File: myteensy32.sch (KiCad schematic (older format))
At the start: 2 parts

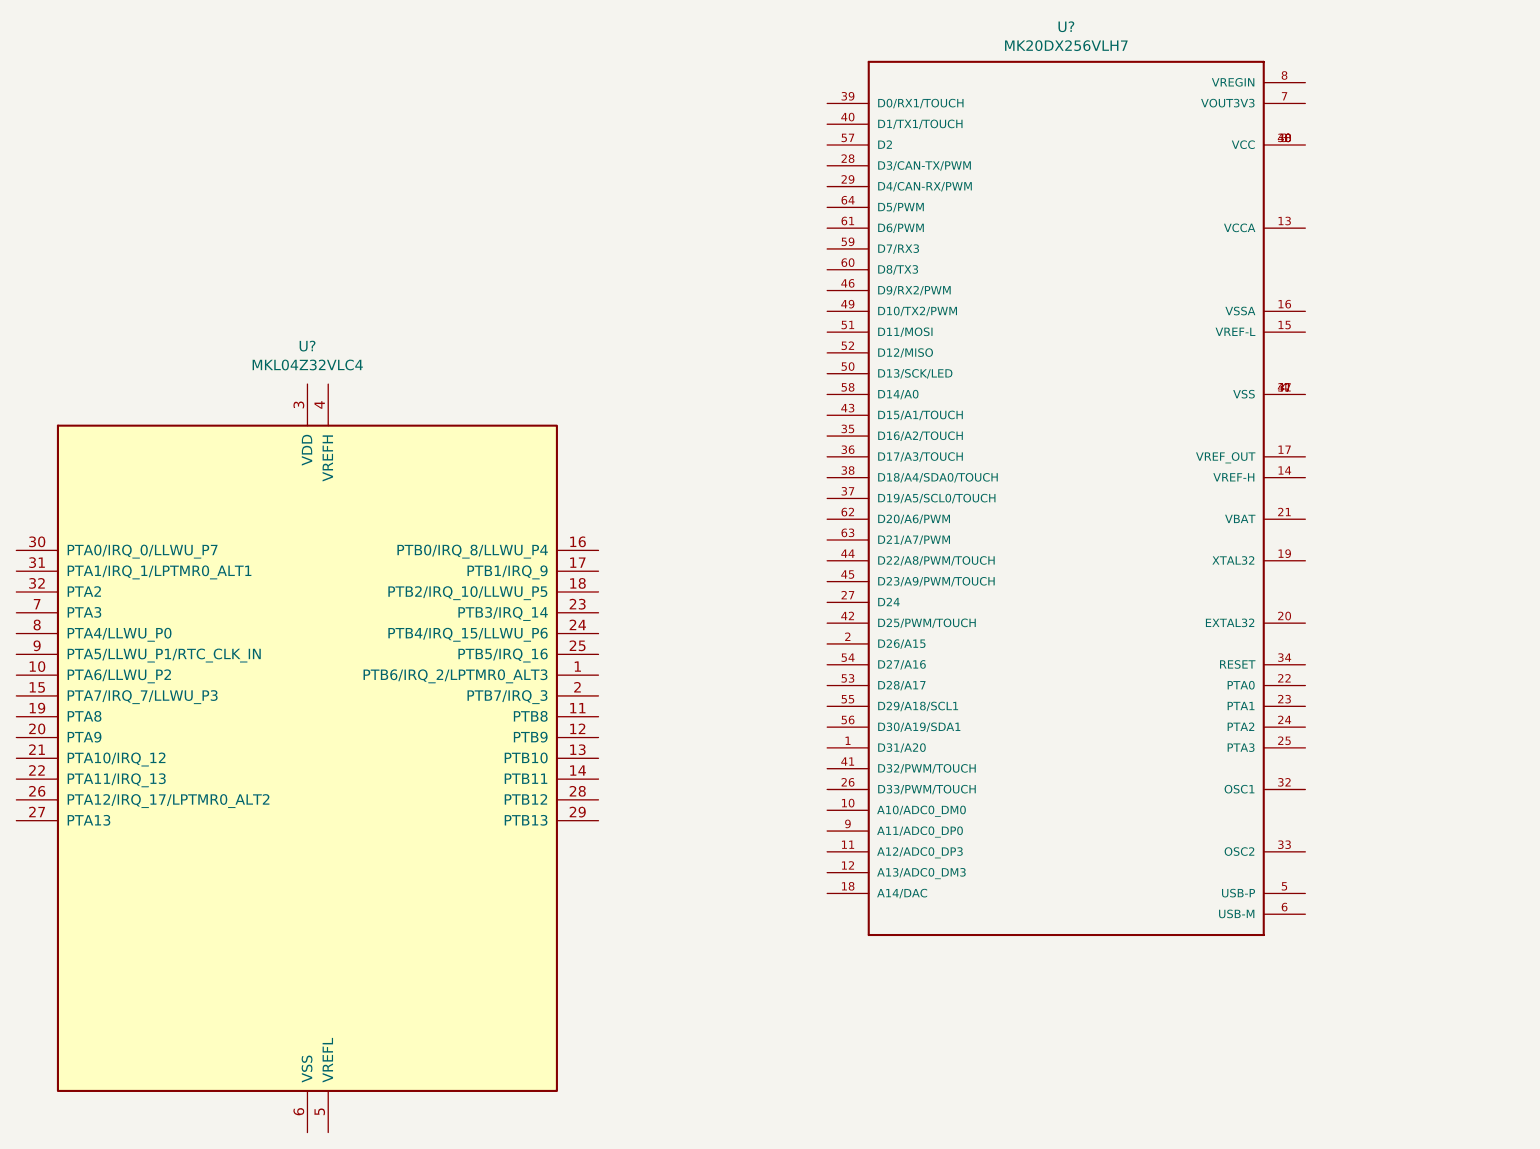
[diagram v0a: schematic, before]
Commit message: シンボルのの作り方が雑だったので心配したけど大丈夫そうだった。
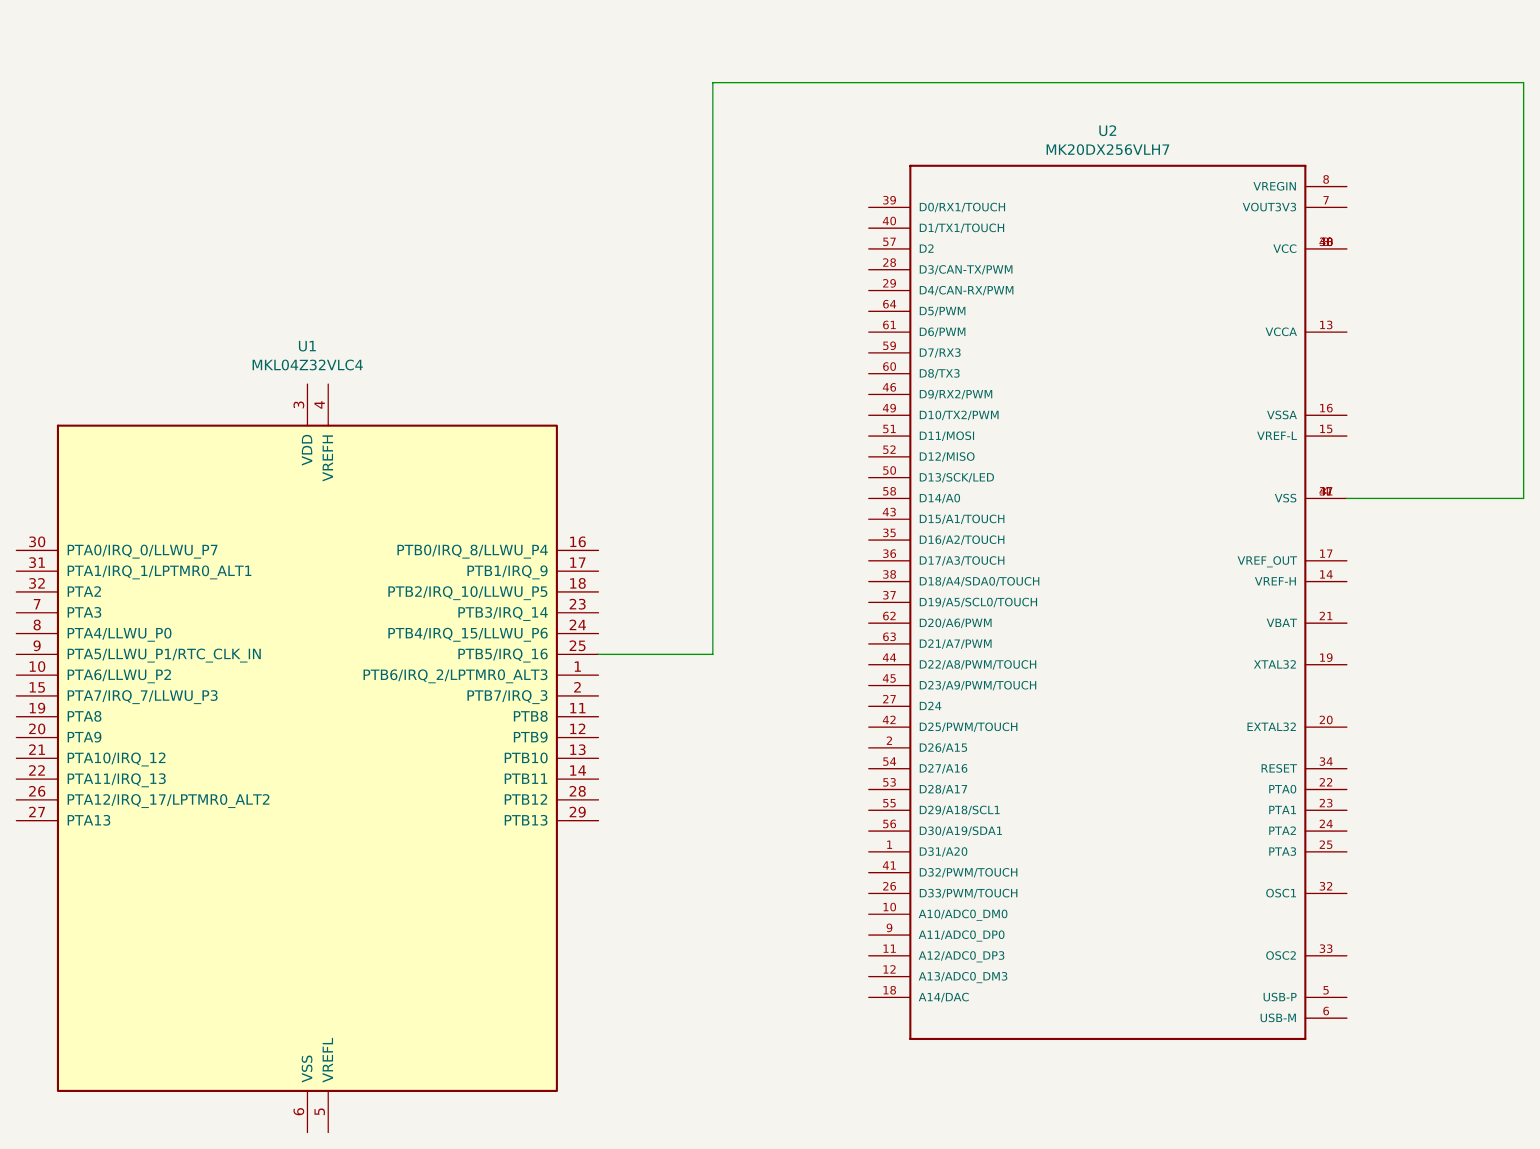
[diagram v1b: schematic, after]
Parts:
- removed U?: MK20DX256VLH7, QFP50P1200X1200X160-64N, symbol mylib:MK20DX256VLH7
- added U2: MK20DX256VLH7, mylib:QFP50P1200X1200X160-64N, symbol mylib:MK20DX256VLH7
- gave numbers to parts that had none: 1
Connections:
- net at U1.25 (PTB5/IRQ_16): now also U2.31 (VSS), U2.4 (VSS), U2.47 (VSS)
- new net: U2.3 (VCC), U2.30 (VCC), U2.48 (VCC)
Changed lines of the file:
@@
 $EndDescr
 $Comp
-L MCU_NXP_Kinetis:MKL04Z32VLC4 U?
+L MCU_NXP_Kinetis:MKL04Z32VLC4 U1
 U 1 1 5F49FA87
 P 4450 4650
-F 0 "U?" H 4450 6631 50  0000 C CNN
+F 0 "U1" H 4450 6631 50  0000 C CNN
 F 1 "MKL04Z32VLC4" H 4450 6540 50  0000 C CNN
 F 2 "Package_QFP:LQFP-32_7x7mm_P0.8mm" H 4600 3025 50  0001 L TNN
@@
 $EndComp
 $Comp
-L mylib:MK20DX256VLH7 U?
-U 1 1 5F4A22C6
-P 8050 3500
-F 0 "U?" H 8100 5867 50  0000 C CNN
-F 1 "MK20DX256VLH7" H 8100 5776 50  0000 C CNN
-F 2 "QFP50P1200X1200X160-64N" H 8050 3500 50  0001 L BNN
-F 3 "" H 8050 3500 50  0001 C CNN
-	1    8050 3500
+L mylib:MK20DX256VLH7 U2
+U 1 1 5F4A610C
+P 8250 4000
+F 0 "U2" H 8300 6367 50  0000 C CNN
+F 1 "MK20DX256VLH7" H 8300 6276 50  0000 C CNN
+F 2 "mylib:QFP50P1200X1200X160-64N" H 8250 4000 50  0001 L BNN
+F 3 "" H 8250 4000 50  0001 C CNN
+	1    8250 4000
 	1    0    0    -1
 $EndComp
+Wire Wire Line
+	9450 3400 10300 3400
+Wire Wire Line
+	10300 3400 10300 1400
+Wire Wire Line
+	10300 1400 6400 1400
+Wire Wire Line
+	6400 4150 5850 4150
+Wire Wire Line
+	6400 1400 6400 4150
 $EndSCHEMATC
